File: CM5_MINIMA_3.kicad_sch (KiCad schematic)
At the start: 18 parts, among them J101 TYPEC-305-ACP16H458, SW101 MK-11C04-G013

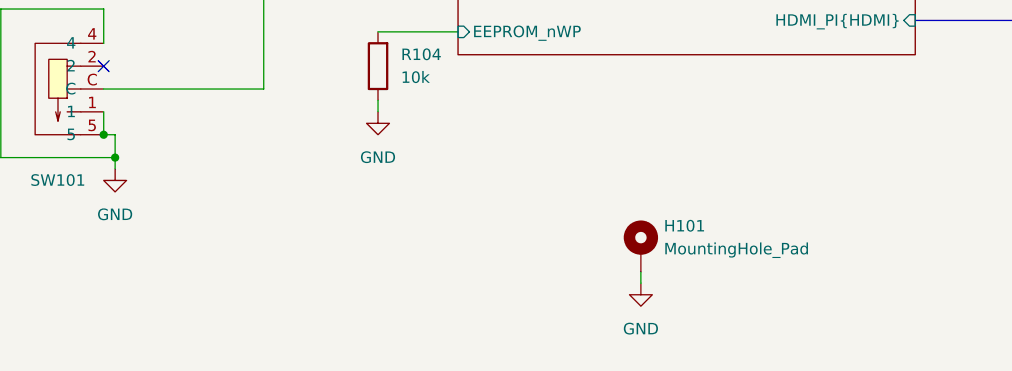
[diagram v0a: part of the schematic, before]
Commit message: arcs
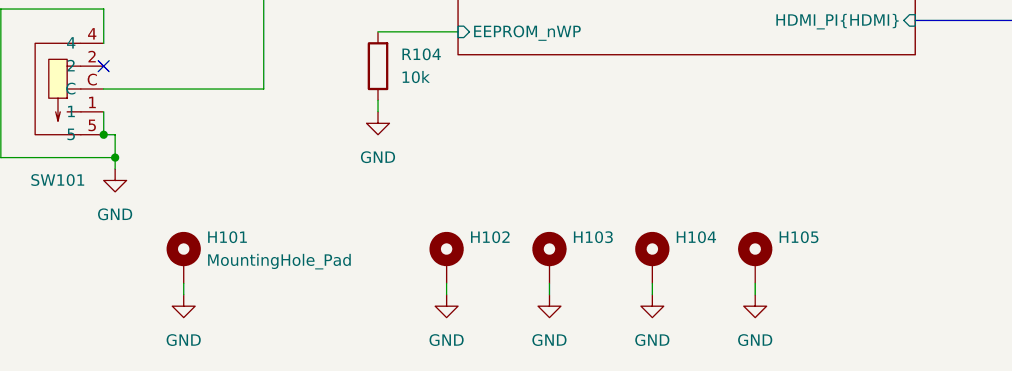
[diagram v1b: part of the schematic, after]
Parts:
- added H102, H103, H104, H105: MountingHole_Pad, MountingHole:MountingHole_2.7mm_Pad, symbol Mechanical:MountingHole_Pad
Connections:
- net GND: now also H102.1, H103.1, H104.1, H105.1
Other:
- moved on the sheet: H101
